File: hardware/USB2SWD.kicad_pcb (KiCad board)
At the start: 2 copper layers, 83.5 x 39 mm, 41 parts, among them J1 USB_C_Receptacle_USB2.0_16P, J2 Conn_01x06_Pin, SW1 SW_SPDT, SW2 PB, U1 STM32F103C8Tx, U2 USBLC6-2P6, U3 FT232RL, U5 W25Q32JVSS, U6 AP2112K-3.3, Y1 Crystal

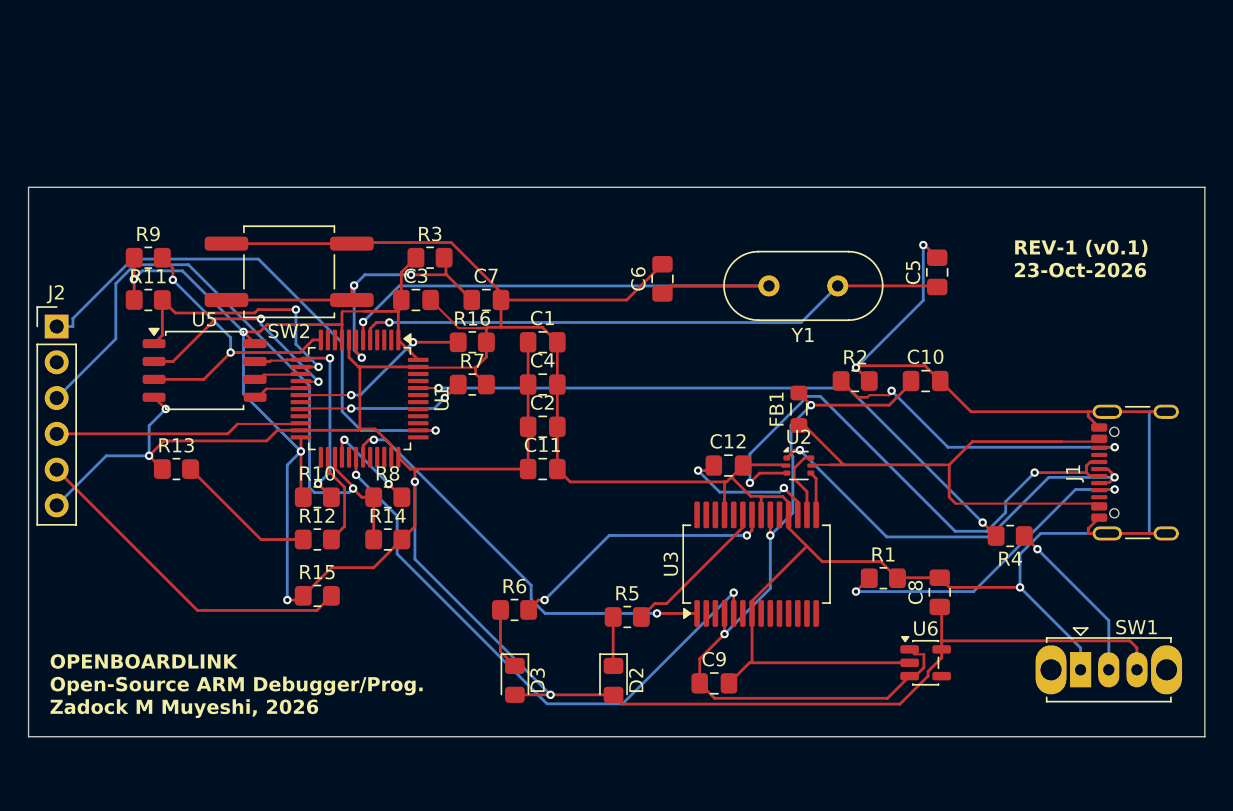
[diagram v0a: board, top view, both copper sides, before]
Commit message: Rev-1 v0.2
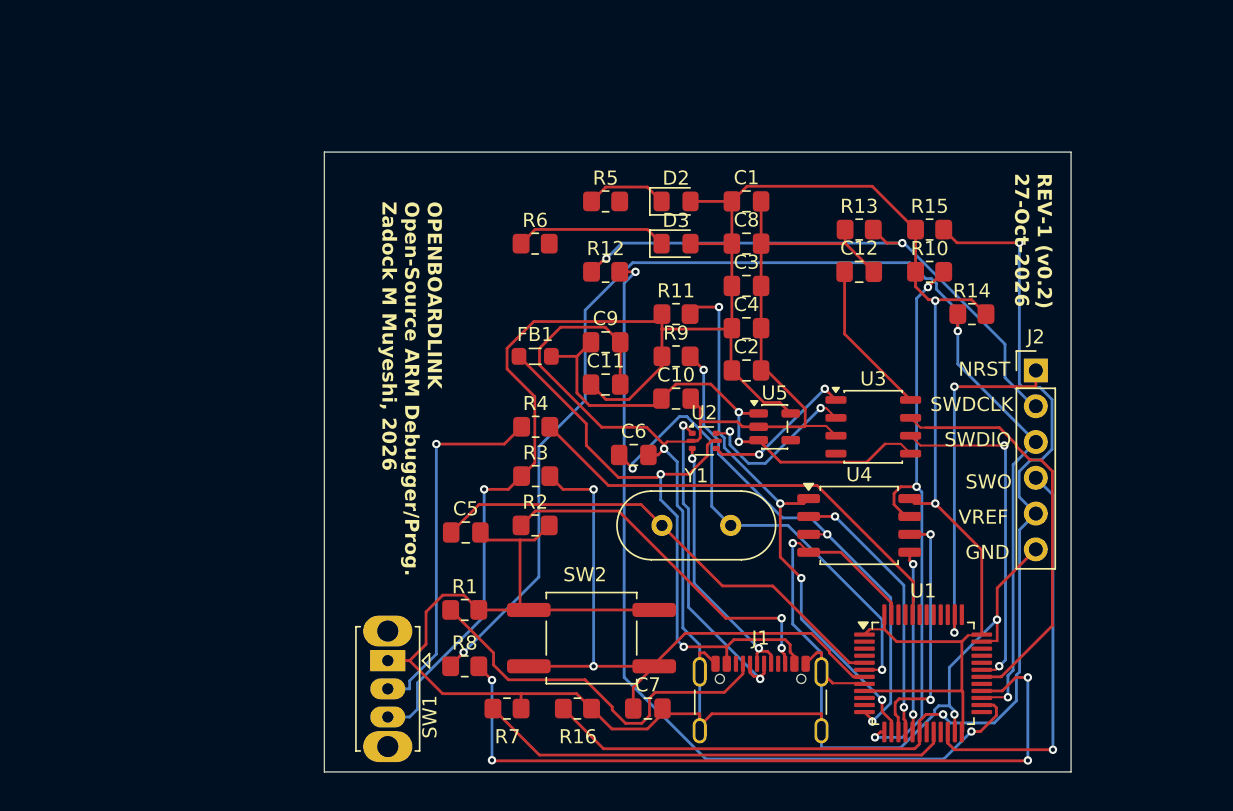
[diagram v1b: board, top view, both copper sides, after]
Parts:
- removed U6: AP2112K-3.3, Package_TO_SOT_SMD:SOT-23-5
- added U4: W25Q32JVSS, Package_SO:SOIC-8_5.3x5.3mm_P1.27mm, F.Cu at (145.5, 112.0)
- U3: value FT232RL -> CH340N; footprint Package_SO:SSOP-28_5.3x10.2mm_P0.65mm -> Package_SO:JEITA_SOIC-8_3.9x4.9mm_P1.27mm
- U5: value W25Q32JVSS -> AP2112K-3.3; footprint Package_SO:SOIC-8_5.3x5.3mm_P1.27mm -> Package_TO_SOT_SMD:SOT-23-5
- moved J2 69.6 mm to (158.0, 101.0)
- moved R13 51.4 mm to (145.5, 91.0)
- moved R15 50.6 mm to (150.5, 91.0)
- moved SW1 49.2 mm to (112.0, 121.6), turned to -90 degrees
- moved R10 46.3 mm to (150.5, 94.0)
- moved U1 44.5 mm to (150.0, 122.5), turned to 0 degrees
- moved R14 44.4 mm to (153.5, 97.0)
- moved U5 40.7 mm to (139.5, 105.0)
- moved C5 38.2 mm to (117.5, 112.5), turned to 0 degrees
- moved R9 38.1 mm to (132.5, 100.0)
- moved R11 37.5 mm to (132.5, 97.0)
- moved R4 34.6 mm to (122.5, 105.0), turned to 0 degrees
- moved D2 34.3 mm to (132.5, 89.0), turned to 0 degrees
- moved SW2 33.7 mm to (126.5, 120.0)
- moved D3 33.0 mm to (132.5, 92.0), turned to 0 degrees
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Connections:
- C12 pad 1: Net-(U3-3V3OUT) -> Net-(U3-V3)
- U3 pad 1: /USART1_RX -> /USB_DP
- U3 pad 2: unconnected-(U3-DTR-Pad2) -> /USB_DM
- U3 pad 3: unconnected-(U3-RTS-Pad3) -> GND
- U3 pad 4: /VBUS -> unconnected-(U3-~{RTS}-Pad4)
- U3 pad 5: /USART1_TX -> /VBUS
- U3 pad 6: unconnected-(U3-RI-Pad6) -> /USART1_RX
- U3 pad 7: GND -> /USART1_TX
- U3 pad 8: (no net) -> Net-(U3-V3)
- U5 pad 1: /SPI1_NSS -> /VBUS
- U5 pad 2: /SPI1_MISO -> GND
- U5 pad 3: /~{FLASH_WP} -> /VBUS
- U5 pad 4: GND -> unconnected-(U5-NC-Pad4)
- U5 pad 5: /SPI1_MOSI -> +3.3V
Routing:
- net /T_SWDCLK: track 6.72 -> 62.0 mm, vias 0 -> 2
- net /SWDIO_IN: track 7.08 -> 54.7 mm, vias 2 -> 4
- net /T_SWDIO: track 45.8 -> 92.4 mm, vias 1 -> 3
- net /VTREF: track 36.8 -> 78.7 mm
- net /T_SWDCLK_P: track 10.1 -> 41.0 mm, vias 0 -> 2
- net GND: track 250.4 -> 219.8 mm, vias 5 -> 4
- net /~{FLASH_HOLD}: track 16.0 -> 41.4 mm, vias 2 -> 3
- net Net-(U1-PB2): track 11.9 -> 33.8 mm, vias 2 -> 0
- net /SPI1_NSS: track 19.3 -> 39.6 mm, vias 2 -> 4
- net Net-(J1-D+-PadA6): track 39.2 -> 18.9 mm
- net /RX_LED: track 19.3 -> 0.00 mm, vias 2 -> 0
- net Net-(U1-NRST): track 27.4 -> 45.9 mm, vias 3 -> 2
- net /VBUS: track 54.5 -> 36.4 mm, vias 3 -> 2
- net /SPI1_SCK: track 3.41 -> 18.1 mm, vias 0 -> 2
- net Net-(SW1-B): track 12.0 -> 26.3 mm
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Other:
- board size 83.5 x 39 mm -> 53 x 44 mm
- board text added: "GND"
- board text added: "NRST"
- board text added: "REV-1 (v0.2) 27-Oct-2026"
- board text added: "SWDCLK"
- board text added: "SWDIO"
- board text added: "SWO"
- board text added: "VREF"
- board text removed: "REV-1 (v0.1) 23-Oct-2026"

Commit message: Rev-1 v0.3
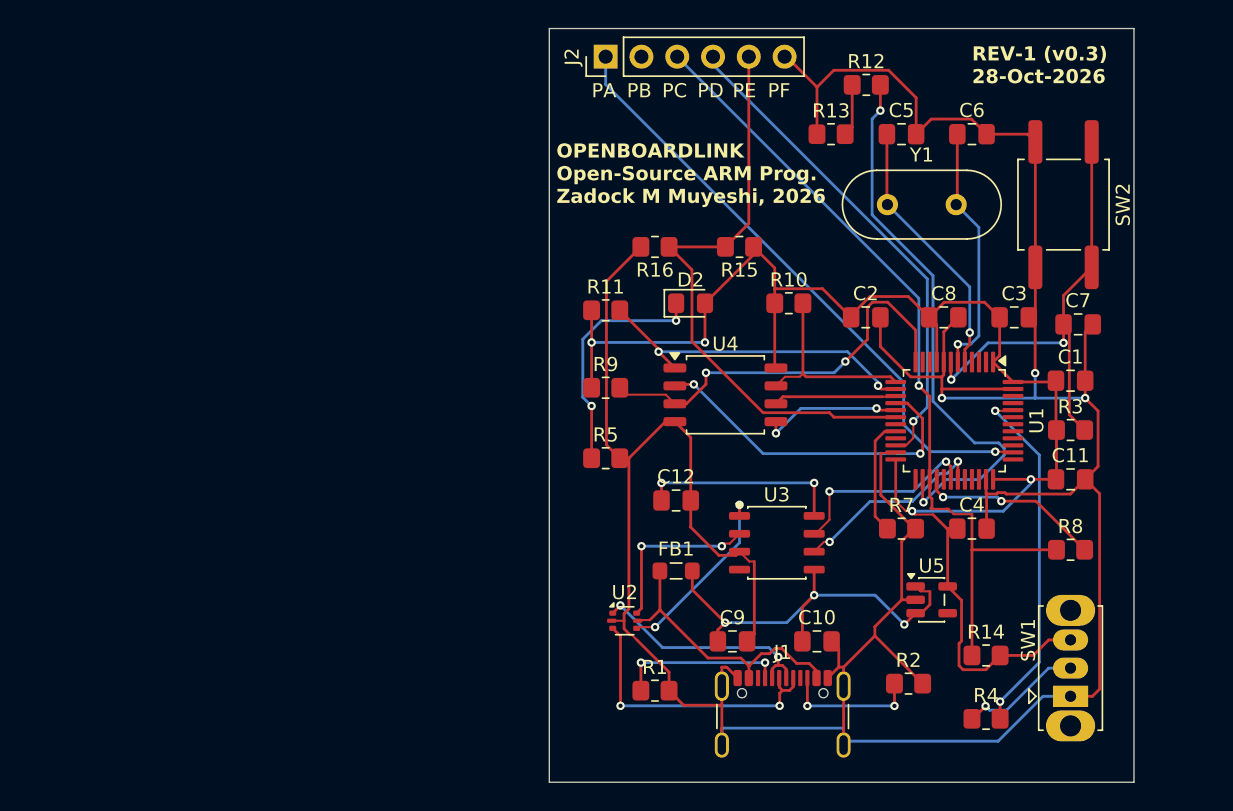
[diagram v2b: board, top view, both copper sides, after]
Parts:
- removed D3: RX LED, LED_SMD:LED_0805_2012Metric_Pad1.15x1.40mm_HandSolder
- removed R6: 1k, Resistor_SMD:R_0805_2012Metric_Pad1.20x1.40mm_HandSolder
- D2: value TX LED -> PWR LED
- moved SW1 48.5 mm to (160.5, 124.1), turned to 90 degrees
- moved SW2 45.5 mm to (160.0, 89.2), turned to 90 degrees
- moved R8 43.8 mm to (160.5, 113.7)
- moved C5 41.9 mm to (148.5, 84.2)
- moved C7 40.9 mm to (161.0, 97.7)
- moved R3 38.1 mm to (160.5, 105.2)
- moved R4 38.1 mm to (154.5, 125.7)
- moved J2 37.8 mm to (127.5, 78.7), turned to 90 degrees
- moved C11 33.7 mm to (160.5, 108.7)
- moved R16 33.2 mm to (131.0, 92.2), turned to 180 degrees
- moved C6 33.1 mm to (153.5, 84.2)
- moved R7 30.8 mm to (148.5, 112.2)
- moved R2 28.8 mm to (149.0, 123.2)
- moved Y1 27.8 mm to (147.5, 89.2)
- moved C1 26.3 mm to (160.5, 101.7)
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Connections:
- R5 pad 2: /TX_LED -> GND
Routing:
- net +3.3V: track 158.6 -> 110.1 mm, vias 3 -> 4
- net /SWDIO_IN: track 54.7 -> 13.0 mm, vias 4 -> 2
- net /T_SWDCLK_P: track 41.0 -> 3.71 mm, vias 2 -> 0
- net /VTREF: track 78.7 -> 42.3 mm, vias 2 -> 0
- net /T_SWDIO: track 92.4 -> 58.7 mm, vias 3 -> 1
- net GND: track 219.8 -> 248.7 mm, vias 4 -> 3
- net /~{FLASH_HOLD}: track 41.4 -> 14.1 mm, vias 3 -> 0
- net Net-(U1-PB2): track 33.8 -> 8.33 mm
- net Net-(U2-VBUS): track 43.6 -> 20.0 mm, vias 2 -> 0
- net /T_SWDCLK: track 62.0 -> 40.2 mm
- net /T_NRST: track 25.7 -> 43.5 mm, vias 2 -> 1
- net Net-(SW1-B): track 26.3 -> 8.73 mm
- net /PD1: track 34.3 -> 18.0 mm, vias 2 -> 1
- net /PD0: track 34.8 -> 18.8 mm, vias 0 -> 1
- net /SPI1_NSS: track 39.6 -> 23.8 mm, vias 4 -> 2
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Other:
- board size 53 x 44 mm -> 41.5 x 53.5 mm
- board text added: "OPENBOARDLINK Open-Source ARM Prog. Zadock M Muyeshi, 2026"
- board text added: "PA"
- board text added: "PA - NRST PB - SWDCLK PC - SWDIO PD - SWO PE - VREF PF - GND"
- board text added: "PB"
- board text added: "PC"
- board text added: "PD"
- board text added: "PE"
- board text added: "PF"
- board text added: "REV-1 (v0.3) 28-Oct-2026"
- board text removed: "GND"
- board text removed: "NRST"
- board text removed: "OPENBOARDLINK Open-Source ARM Debugger/Prog. Zadock M Muyeshi, 2026"
- board text removed: "REV-1 (v0.2) 27-Oct-2026"
- board text removed: "SWDCLK"
- board text removed: "SWDIO"
- board text removed: "SWO"
- board text removed: "VREF"
